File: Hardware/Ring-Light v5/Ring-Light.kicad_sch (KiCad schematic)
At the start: 21 parts, among them J1 694106301002, J5 640445-2, Q1 PMOS, U36 TPS62177DQC

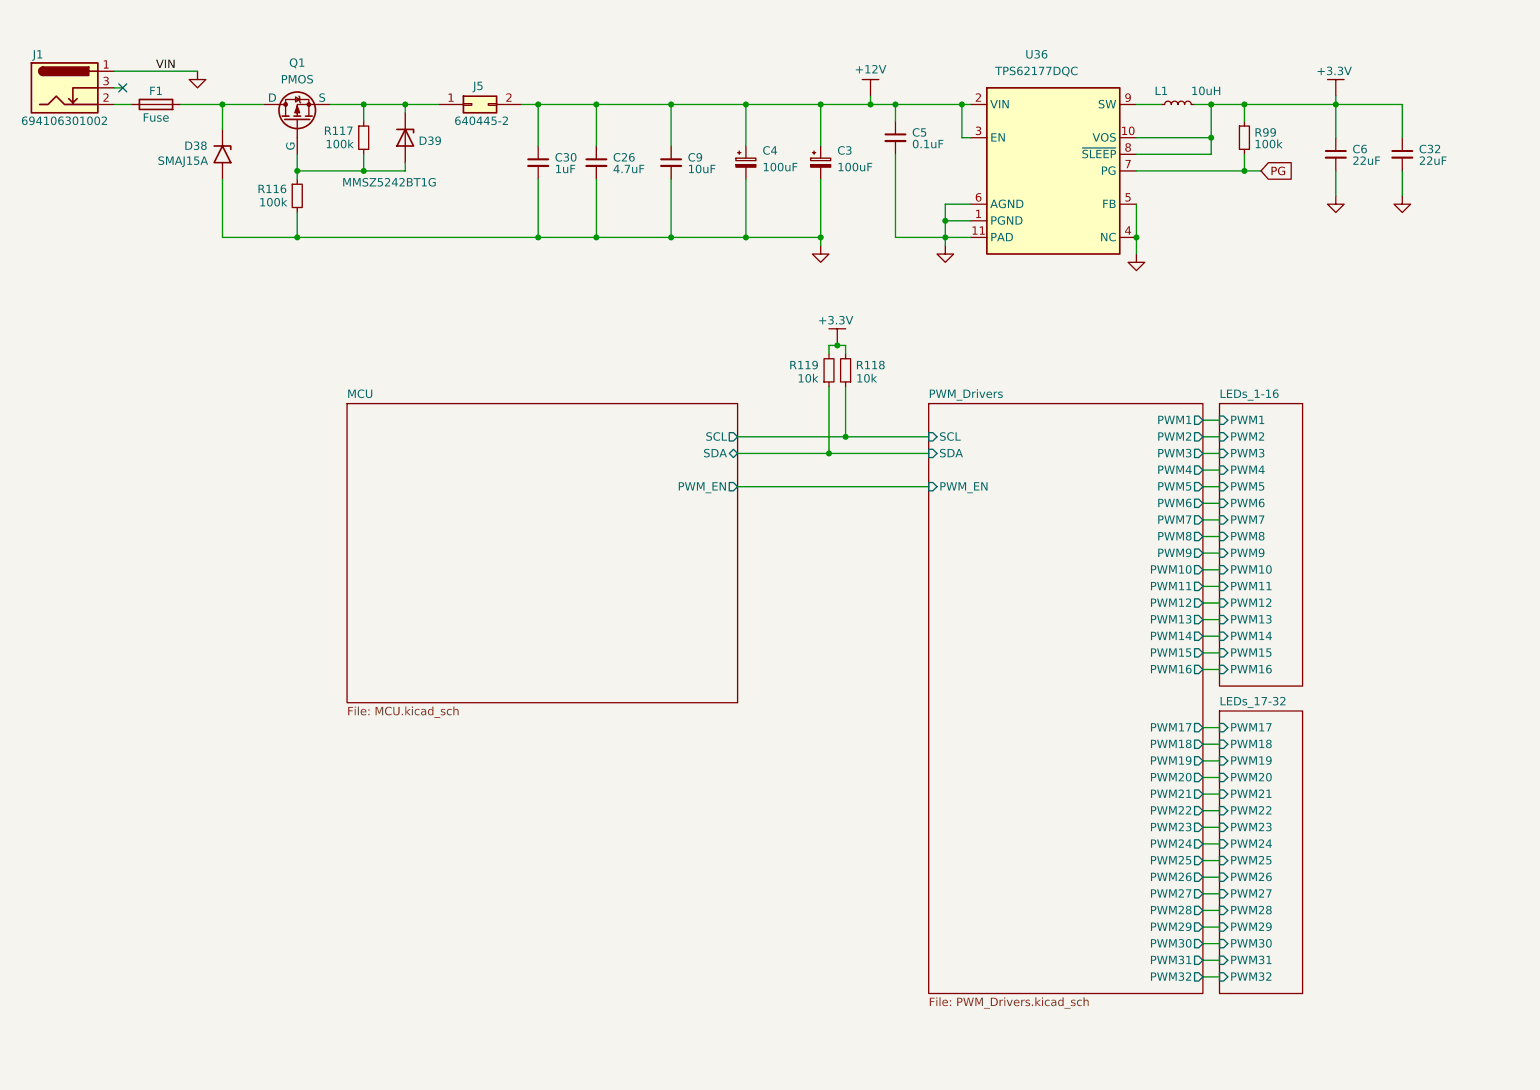
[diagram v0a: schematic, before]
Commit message: m
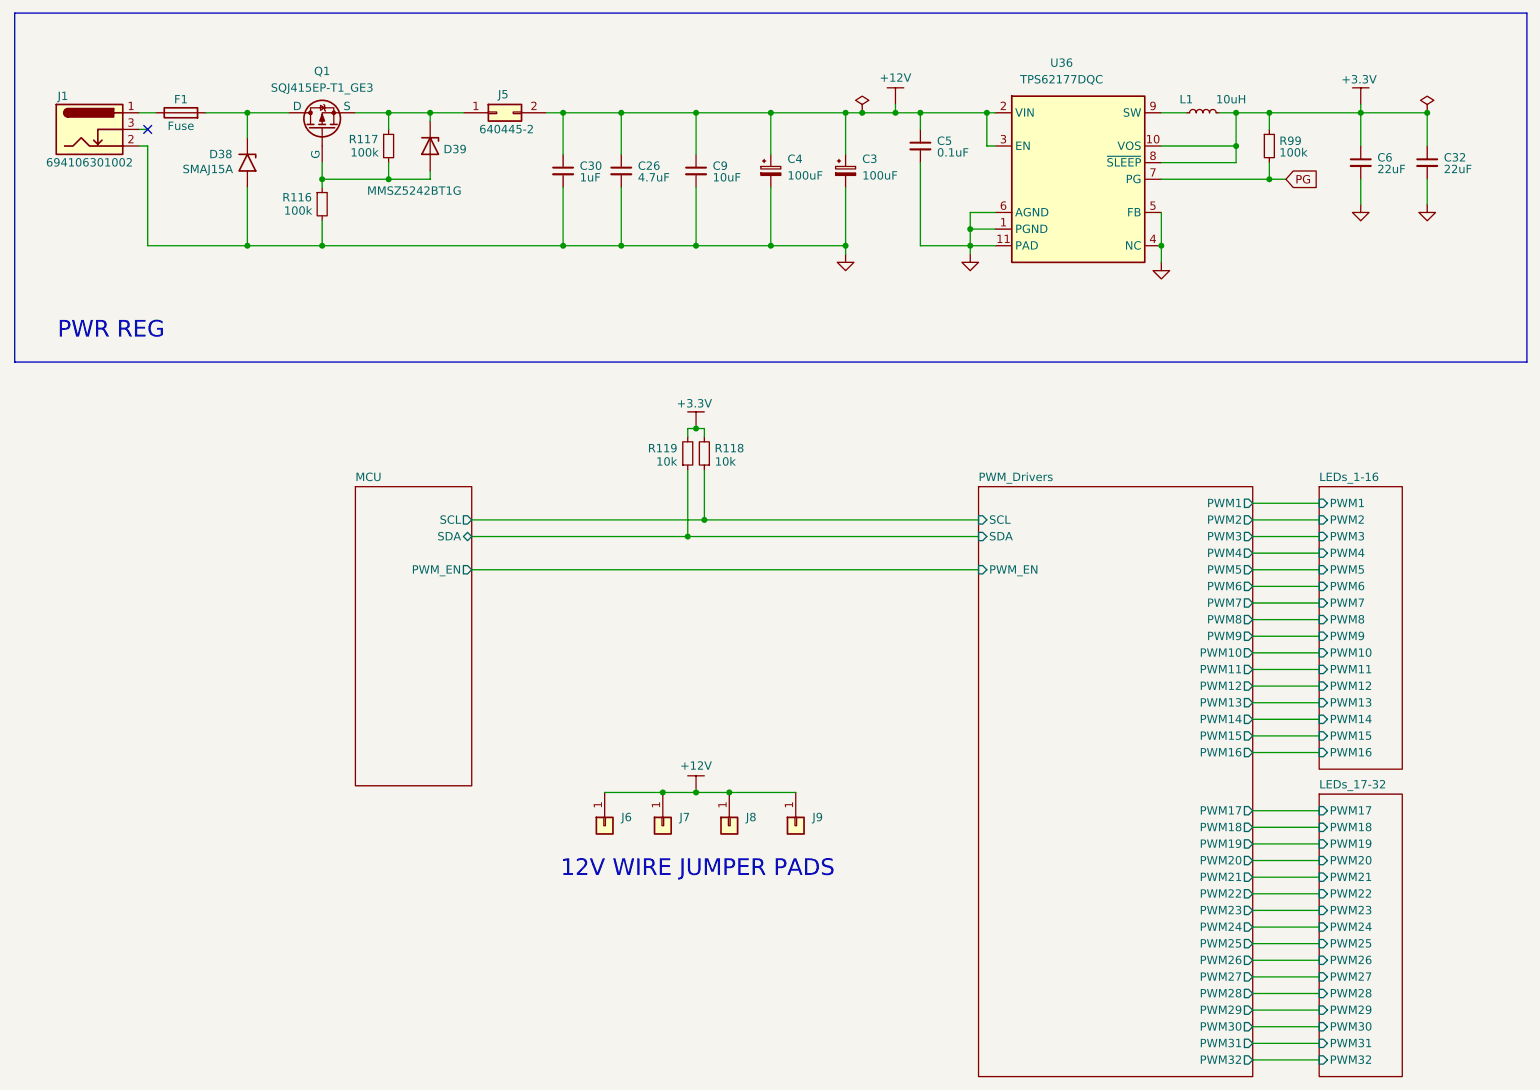
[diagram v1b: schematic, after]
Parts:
- removed Q1: PMOS, symbol Simulation_SPICE:PMOS
- added J6, J7, J8, J9: Conn_01x01, symbol Connector_Generic:Conn_01x01
- added Q1: SQJ415EP-T1_GE3, Library:SOT_SQJ415EP_VIS, symbol Library:PMOS
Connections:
- net +12V: now also J6.1 (Pin_1), J7.1 (Pin_1), J8.1 (Pin_1), J9.1 (Pin_1)
- net GND: now also J1.2; no longer J1.1
- net at D38.1 (A1), F1.2: now also Q1.5 (D)
- net at F1.1: now also J1.1; no longer J1.2
- net at D39.1 (K), J5.1 (Pin_1), R117.1: now also Q1.1 (S), Q1.2 (S), Q1.3 (S)
- net at D39.2 (A), R116.1, R117.2: now also Q1.4 (G)
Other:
- note added: "12V WIRE JUMPER PADS"
- note added: "PWR REG"
- moved on the sheet: C26, C3, C30, C32, C4, C5, C6, C9, D38, D39, F1, J1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
